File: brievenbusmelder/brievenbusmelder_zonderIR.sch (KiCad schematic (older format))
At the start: 14 parts, among them IC3 VCNL4035X01-GS08, J4 Conn_01x05_Male

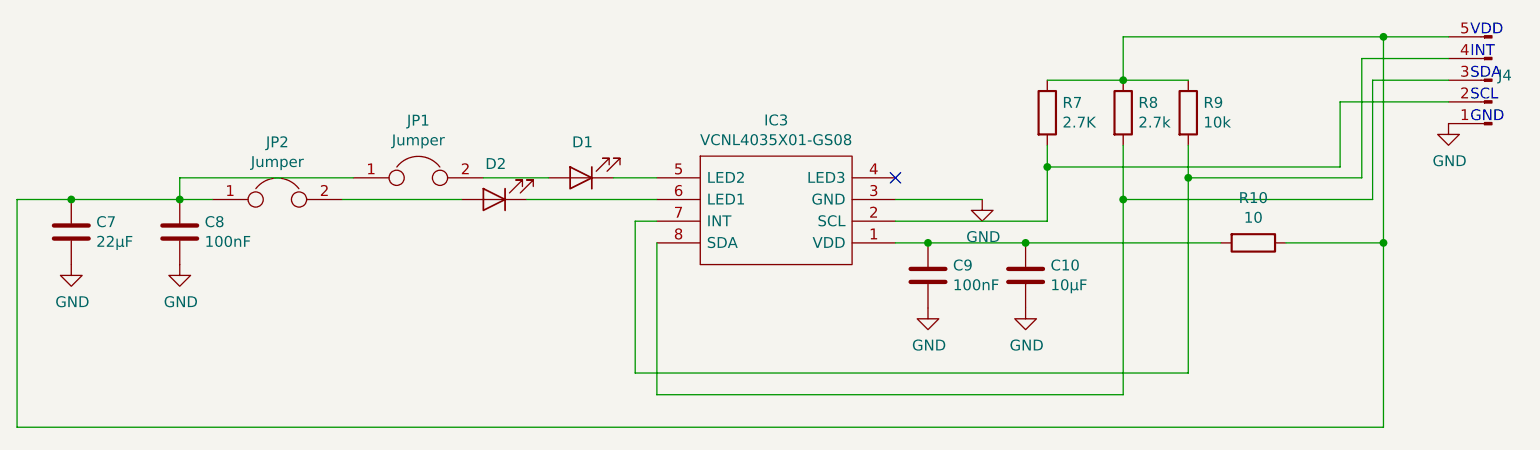
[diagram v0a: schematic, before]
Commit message: Update brievenbusmelder_zonderIR.sch
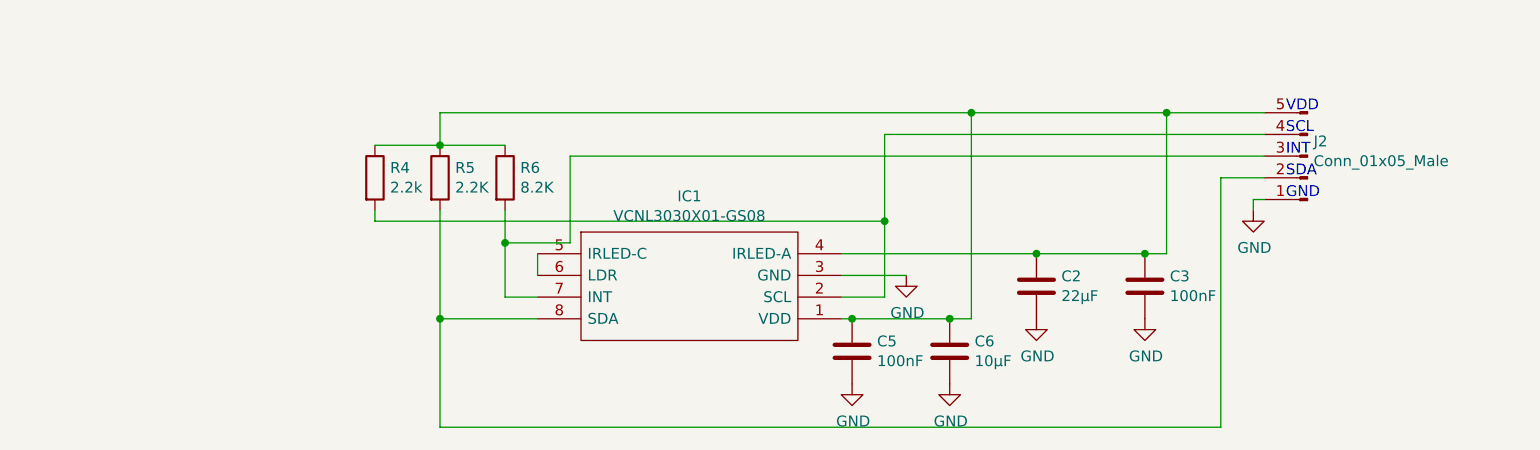
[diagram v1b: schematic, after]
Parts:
- removed C10: 10µF, Capacitor_SMD:C_1206_3216Metric_Pad1.42x1.75mm_HandSolder, symbol Device:C
- removed C7: 22µF, Capacitor_SMD:C_1206_3216Metric_Pad1.42x1.75mm_HandSolder, symbol Device:C
- removed C8, C9: 100nF, Capacitor_SMD:C_1206_3216Metric_Pad1.42x1.75mm_HandSolder, symbol Device:C
- removed D1: IR, LED_SMD:LED_1206_3216Metric_Pad1.42x1.75mm_HandSolder, symbol Device:LED
- removed D2: IR, IR_TH:OP294, symbol Device:LED
- removed IC3: VCNL4035X01-GS08, naderingssensor_zonderIR:naderingssensor_zonderIR, symbol lichtsensor:VCNL4035X01-GS08
- removed J4: Conn_01x05_Male, Connector_PinHeader_2.54mm:PinHeader_1x05_P2.54mm_Vertical, symbol Connector:Conn_01x05_Male
- removed JP1, JP2: Jumper, Connector_PinHeader_2.54mm:PinHeader_1x02_P2.54mm_Vertical, symbol Device:Jumper
- removed R10: 10, Resistor_SMD:R_1206_3216Metric_Pad1.42x1.75mm_HandSolder, symbol Device:R
- removed R7: 2.7K, Resistor_SMD:R_1206_3216Metric_Pad1.42x1.75mm_HandSolder, symbol Device:R
- removed R8: 2.7k, Resistor_SMD:R_1206_3216Metric_Pad1.42x1.75mm_HandSolder, symbol Device:R
- removed R9: 10k, Resistor_SMD:R_1206_3216Metric_Pad1.42x1.75mm_HandSolder, symbol Device:R
- added C2: 22µF, Capacitor_SMD:C_1206_3216Metric_Pad1.42x1.75mm_HandSolder, symbol Device:C
- added C3, C5: 100nF, Capacitor_SMD:C_1206_3216Metric_Pad1.42x1.75mm_HandSolder, symbol Device:C
- added C6: 10µF, Capacitor_SMD:C_1206_3216Metric_Pad1.42x1.75mm_HandSolder, symbol Device:C
- added IC1: VCNL3030X01-GS08, naderingssensor_metIR:VCNL3030X01GS08, symbol naderingssensor:VCNL3030X01-GS08
- added J2: Conn_01x05_Male, Connector_PinHeader_2.54mm:PinHeader_1x05_P2.54mm_Vertical, symbol Connector:Conn_01x05_Male
- added R4: 2.2k, Resistor_SMD:R_1206_3216Metric_Pad1.42x1.75mm_HandSolder, symbol Device:R
- added R5: 2.2K, Resistor_SMD:R_1206_3216Metric_Pad1.42x1.75mm_HandSolder, symbol Device:R
- added R6: 8.2K, Resistor_SMD:R_1206_3216Metric_Pad1.42x1.75mm_HandSolder, symbol Device:R
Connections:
- net GND: now also C2.2, C3.2, C5.2, C6.2, IC1.3 (GND), J2.1 (Pin_1)
- new net: C2.1, C3.1, C5.1, C6.1, IC1.1 (VDD), IC1.4 (IRLED-A), J2.5 (Pin_5), R4.1, R5.1, R6.1
- new net: IC1.2 (SCL), J2.4 (Pin_4), R4.2
- new net: IC1.5 (IRLED-C), IC1.6 (LDR)
- new net: IC1.7 (INT), J2.3 (Pin_3), R6.2
- new net: IC1.8 (SDA), J2.2 (Pin_2), R5.2
- no-connect marks 1 -> 0
